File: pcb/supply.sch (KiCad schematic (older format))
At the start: 19 parts, among them J13 Conn_01x02_Female, U18 ZLDO1117G33TA, U19 ZLDO1117G12TA, U9 ZLDO1117G33TA

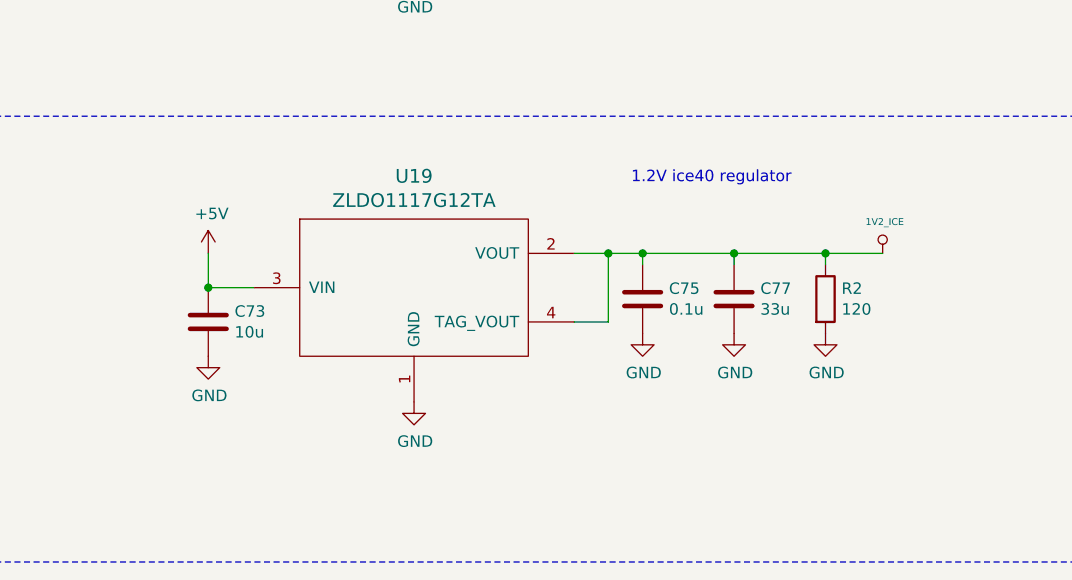
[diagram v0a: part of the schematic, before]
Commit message: small 1.2V reg
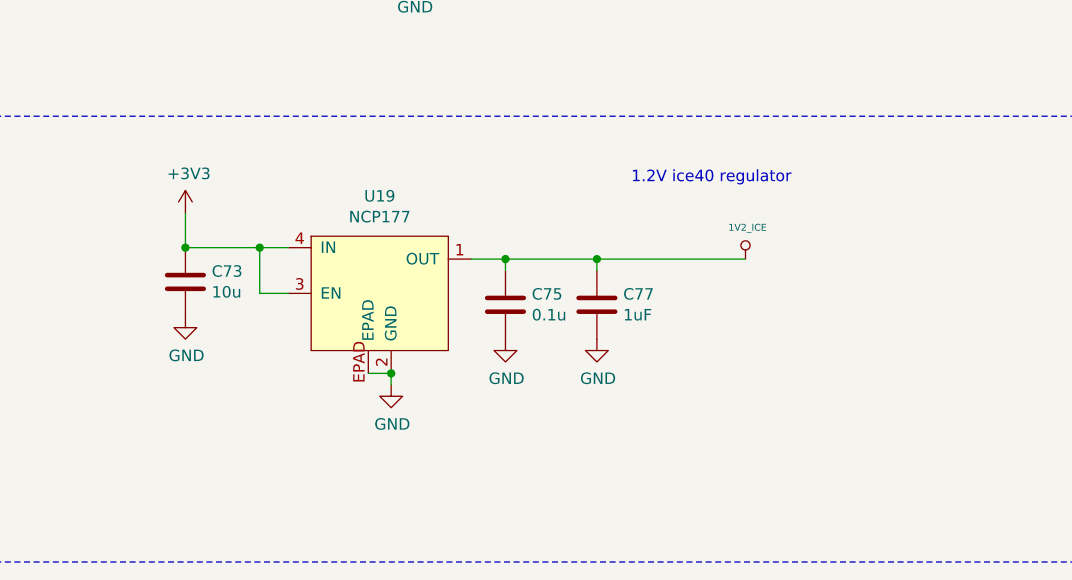
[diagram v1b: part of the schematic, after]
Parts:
- removed R2: 120, Resistor_SMD:R_0402_1005Metric, symbol Device:R
- removed U19: ZLDO1117G12TA, symbol ZLDO1117G33TA:ZLDO1117G12TA
- added U19: NCP177, SMD:XDFN4, symbol ncp177:NCP177
- C73: footprint Capacitor_SMD:C_0805_2012Metric -> Capacitor_SMD:C_0603_1608Metric
- C75: footprint Capacitor_SMD:C_0603_1608Metric -> Capacitor_SMD:C_0402_1005Metric
- C77: value 33u -> 1uF; footprint Capacitor_SMD:C_1206_3216Metric -> Capacitor_SMD:C_0603_1608Metric
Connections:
- net +5V: no longer C73.1
- net 1V2_ICE: now also U19.1 (OUT)
- net GND: now also U19.2 (GND), U19.EPAD
- new net +3V3: C73.1, U19.3 (EN), U19.4 (IN)
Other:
- moved on the sheet: C73, C75, C77
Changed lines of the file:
@@
 	6300 450  6300 6300
-$Comp
-L power:+5V #PWR0225
-U 1 1 5EA0A264
-P 7400 4950
-F 0 "#PWR0225" H 7400 4800 50  0001 C CNN
-F 1 "+5V" H 7415 5123 50  0000 C CNN
-F 2 "" H 7400 4950 50  0001 C CNN
-F 3 "" H 7400 4950 50  0001 C CNN
-	1    7400 4950
-	1    0    0    -1
-$EndComp
-$Comp
-L power:GND #PWR0226
-U 1 1 5EA0A26E
-P 8300 5600
-F 0 "#PWR0226" H 8300 5350 50  0001 C CNN
-F 1 "GND" H 8305 5427 50  0000 C CNN
-F 2 "" H 8300 5600 50  0001 C CNN
-F 3 "" H 8300 5600 50  0001 C CNN
-	1    8300 5600
-	1    0    0    -1
-$EndComp
-Wire Wire Line
-	9000 5250 9150 5250
-Wire Wire Line
-	9150 5250 9150 4950
-Wire Wire Line
-	9150 4950 9000 4950
-Wire Wire Line
-	10350 4950 10100 4950
-Connection ~ 9150 4950
 $Comp
 L Device:C C75
 U 1 1 5EA0A27E
-P 9300 5150
-F 0 "C75" H 9415 5196 50  0000 L CNN
-F 1 "0.1u" H 9415 5105 50  0000 L CNN
-F 2 "Capacitor_SMD:C_0603_1608Metric" H 9338 5000 50  0001 C CNN
-F 3 "~" H 9300 5150 50  0001 C CNN
-F 4 "720-1688-1-ND" H 9300 5150 50  0001 C CNN "DigiKey"
-	1    9300 5150
+P 8700 5175
+F 0 "C75" H 8815 5221 50  0000 L CNN
+F 1 "0.1u" H 8815 5130 50  0000 L CNN
+F 2 "Capacitor_SMD:C_0402_1005Metric" H 8738 5025 50  0001 C CNN
+F 3 "~" H 8700 5175 50  0001 C CNN
+F 4 "720-1688-1-ND" H 8700 5175 50  0001 C CNN "DigiKey"
+	1    8700 5175
 	1    0    0    -1
 $EndComp
@@
 L Device:C C77
 U 1 1 5EA0A289
-P 9700 5150
-F 0 "C77" H 9815 5196 50  0000 L CNN
-F 1 "33u" H 9815 5105 50  0000 L CNN
-F 2 "Capacitor_SMD:C_1206_3216Metric" H 9738 5000 50  0001 C CNN
-F 3 "~" H 9700 5150 50  0001 C CNN
-F 4 "445-14751-1-ND" H 9700 5150 50  0001 C CNN "DigiKey"
-	1    9700 5150
+P 9100 5175
+F 0 "C77" H 9215 5221 50  0000 L CNN
+F 1 "1uF" H 9215 5130 50  0000 L CNN
+F 2 "Capacitor_SMD:C_0603_1608Metric" H 9138 5025 50  0001 C CNN
+F 3 "~" H 9100 5175 50  0001 C CNN
+F 4 "445-14751-1-ND" H 9100 5175 50  0001 C CNN "DigiKey"
+	1    9100 5175
 	1    0    0    -1
 $EndComp
@@
 L Device:C C73
 U 1 1 5EA0A294
-P 7400 5250
-F 0 "C73" H 7515 5296 50  0000 L CNN
-F 1 "10u" H 7515 5205 50  0000 L CNN
-F 2 "Capacitor_SMD:C_0805_2012Metric" H 7438 5100 50  0001 C CNN
-F 3 "~" H 7400 5250 50  0001 C CNN
-F 4 "1276-6456-1-ND" H 7400 5250 50  0001 C CNN "DigiKey"
-	1    7400 5250
+P 7300 5075
+F 0 "C73" H 7415 5121 50  0000 L CNN
+F 1 "10u" H 7415 5030 50  0000 L CNN
+F 2 "Capacitor_SMD:C_0603_1608Metric" H 7338 4925 50  0001 C CNN
+F 3 "~" H 7300 5075 50  0001 C CNN
+F 4 "1276-6456-1-ND" H 7300 5075 50  0001 C CNN "DigiKey"
+	1    7300 5075
 	1    0    0    -1
 $EndComp
 Wire Wire Line
-	7600 5100 7400 5100
+	7300 4775 7300 4925
+Connection ~ 7300 4925
 Wire Wire Line
-	7400 4950 7400 5100
-Connection ~ 7400 5100
+	8700 5025 8700 4975
+Connection ~ 8700 4975
 Wire Wire Line
-	9300 5000 9300 4950
-Connection ~ 9300 4950
+	8700 4975 8550 4975
 Wire Wire Line
-	9300 4950 9150 4950
+	9100 5025 9100 4975
+Connection ~ 9100 4975
 Wire Wire Line
-	9700 5000 9700 4950
-Connection ~ 9700 4950
-Wire Wire Line
-	9700 4950 9300 4950
+	9100 4975 8700 4975
 $Comp
 L power:GND #PWR0227
 U 1 1 5EA0A2A7
-P 7400 5400
-F 0 "#PWR0227" H 7400 5150 50  0001 C CNN
-F 1 "GND" H 7405 5227 50  0000 C CNN
-F 2 "" H 7400 5400 50  0001 C CNN
-F 3 "" H 7400 5400 50  0001 C CNN
-	1    7400 5400
+P 7300 5225
+F 0 "#PWR0227" H 7300 4975 50  0001 C CNN
+F 1 "GND" H 7305 5052 50  0000 C CNN
+F 2 "" H 7300 5225 50  0001 C CNN
+F 3 "" H 7300 5225 50  0001 C CNN
+	1    7300 5225
 	1    0    0    -1
 $EndComp
@@
 L power:GND #PWR0228
 U 1 1 5EA0A2B1
-P 9300 5300
-F 0 "#PWR0228" H 9300 5050 50  0001 C CNN
-F 1 "GND" H 9305 5127 50  0000 C CNN
-F 2 "" H 9300 5300 50  0001 C CNN
-F 3 "" H 9300 5300 50  0001 C CNN
-	1    9300 5300
+P 8700 5325
+F 0 "#PWR0228" H 8700 5075 50  0001 C CNN
+F 1 "GND" H 8705 5152 50  0000 C CNN
+F 2 "" H 8700 5325 50  0001 C CNN
+F 3 "" H 8700 5325 50  0001 C CNN
+	1    8700 5325
 	1    0    0    -1
 $EndComp
@@
 L power:GND #PWR0229
 U 1 1 5EA0A2BB
-P 9700 5300
-F 0 "#PWR0229" H 9700 5050 50  0001 C CNN
-F 1 "GND" H 9705 5127 50  0000 C CNN
-F 2 "" H 9700 5300 50  0001 C CNN
-F 3 "" H 9700 5300 50  0001 C CNN
-	1    9700 5300
+P 9100 5325
+F 0 "#PWR0229" H 9100 5075 50  0001 C CNN
+F 1 "GND" H 9105 5152 50  0000 C CNN
+F 2 "" H 9100 5325 50  0001 C CNN
+F 3 "" H 9100 5325 50  0001 C CNN
+	1    9100 5325
 	1    0    0    -1
 $EndComp
@@
 L ventilator-PowerSymbols:1V2_ICE #PWR0230
 U 1 1 5EA0EA1D
-P 10350 4950
-F 0 "#PWR0230" H 10350 4910 30  0001 C CNN
-F 1 "1V2_ICE" H 10359 5088 30  0000 C CNN
-F 2 "" H 10350 4950 60  0000 C CNN
-F 3 "" H 10350 4950 60  0000 C CNN
-	1    10350 4950
+P 9750 4975
+F 0 "#PWR0230" H 9750 4935 30  0001 C CNN
+F 1 "1V2_ICE" H 9759 5113 30  0000 C CNN
+F 2 "" H 9750 4975 60  0000 C CNN
+F 3 "" H 9750 4975 60  0000 C CNN
+	1    9750 4975
 	1    0    0    -1
 $EndComp
 $Comp
-L ZLDO1117G33TA:ZLDO1117G12TA U19
-U 1 1 5EA0F149
-P 8300 5100
-F 0 "U19" H 8300 5587 60  0000 C CNN
-F 1 "ZLDO1117G12TA" H 8300 5481 60  0000 C CNN
-F 2 "" H 8450 5150 60  0000 C CNN
-F 3 "" H 8450 5150 60  0000 C CNN
-	1    8300 5100
+L ncp177:NCP177 U19
+U 1 1 5EA22602
+P 8150 5125
+F 0 "U19" H 8150 5550 50  0000 C CNN
+F 1 "NCP177" H 8150 5459 50  0000 C CNN
+F 2 "SMD:XDFN4" H 7900 5425 50  0001 C CNN
+F 3 "" H 7900 5425 50  0001 C CNN
+	1    8150 5125
+	1    0    0    -1
+$EndComp
+Wire Wire Line
+	9100 4975 9750 4975
+Wire Wire Line
+	7300 4925 7625 4925
+Wire Wire Line
+	7625 5125 7625 4925
+Connection ~ 7625 4925
+Wire Wire Line
+	7625 4925 7750 4925
+Wire Wire Line
+	7625 5125 7750 5125
+$Comp
+L power:+3V3 #PWR0225
+U 1 1 5EA2F978
+P 7300 4775
+F 0 "#PWR0225" H 7300 4625 50  0001 C CNN
+F 1 "+3V3" H 7315 4948 50  0000 C CNN
+F 2 "" H 7300 4775 50  0001 C CNN
+F 3 "" H 7300 4775 50  0001 C CNN
+	1    7300 4775
 	1    0    0    -1
 $EndComp
 $Comp
-L Device:R R2
-U 1 1 5EA113A0
-P 10100 5150
-F 0 "R2" H 10170 5196 50  0000 L CNN
-F 1 "120" H 10170 5105 50  0000 L CNN
-F 2 "Resistor_SMD:R_0402_1005Metric" V 10030 5150 50  0001 C CNN
-F 3 "~" H 10100 5150 50  0001 C CNN
-	1    10100 5150
+L power:GND #PWR0226
+U 1 1 5EA31ABA
+P 8200 5525
+F 0 "#PWR0226" H 8200 5275 50  0001 C CNN
+F 1 "GND" H 8205 5352 50  0000 C CNN
+F 2 "" H 8200 5525 50  0001 C CNN
+F 3 "" H 8200 5525 50  0001 C CNN
+	1    8200 5525
 	1    0    0    -1
 $EndComp
 Wire Wire Line
-	10100 5000 10100 4950
-Connection ~ 10100 4950
+	8100 5475 8200 5475
 Wire Wire Line
-	10100 4950 9700 4950
-$Comp
-L power:GND #PWR0231
-U 1 1 5EA127C0
-P 10100 5300
-F 0 "#PWR0231" H 10100 5050 50  0001 C CNN
-F 1 "GND" H 10105 5127 50  0000 C CNN
-F 2 "" H 10100 5300 50  0001 C CNN
-F 3 "" H 10100 5300 50  0001 C CNN
-	1    10100 5300
-	1    0    0    -1
-$EndComp
+	8200 5475 8200 5525
+Connection ~ 8200 5475
 $EndSCHEMATC
